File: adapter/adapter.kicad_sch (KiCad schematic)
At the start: 13 parts, among them J1 AudioJack4, J2 AudioJack4, J3 Conn_01x02_Female, J4 Conn_01x03_Female, J5 Conn_01x03_Female, J6 Conn_01x02_Female, J7 Conn_01x06_Female, J9 Conn_01x06_Female, SW1 SW_SPST, SW2 SW_SPST, U1 eliteC, U2 eliteC, U3 YAAJ_WeAct_BlackPill_Part_Lik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

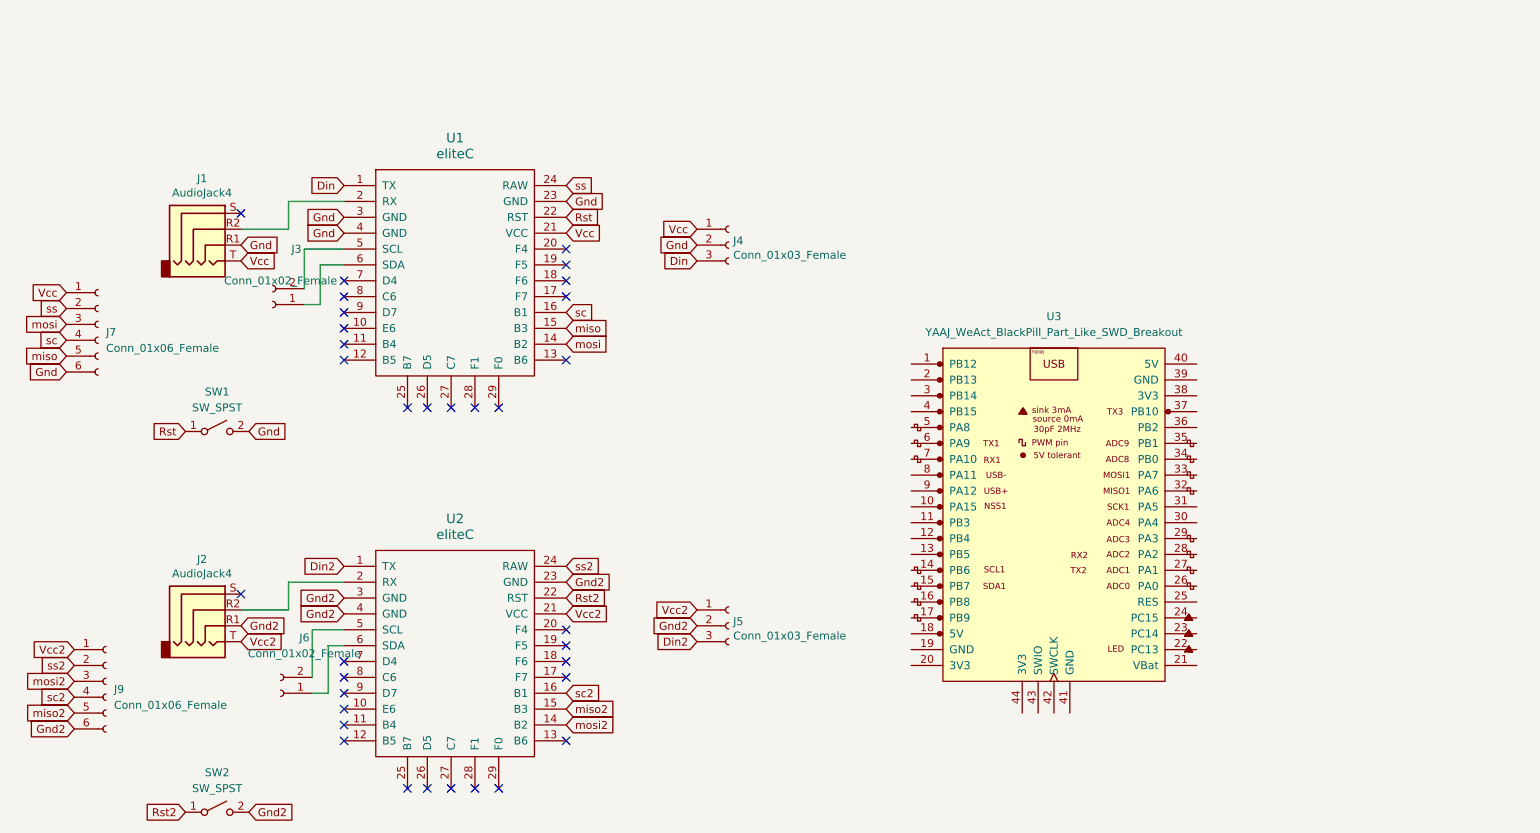
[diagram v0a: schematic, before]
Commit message: pinout
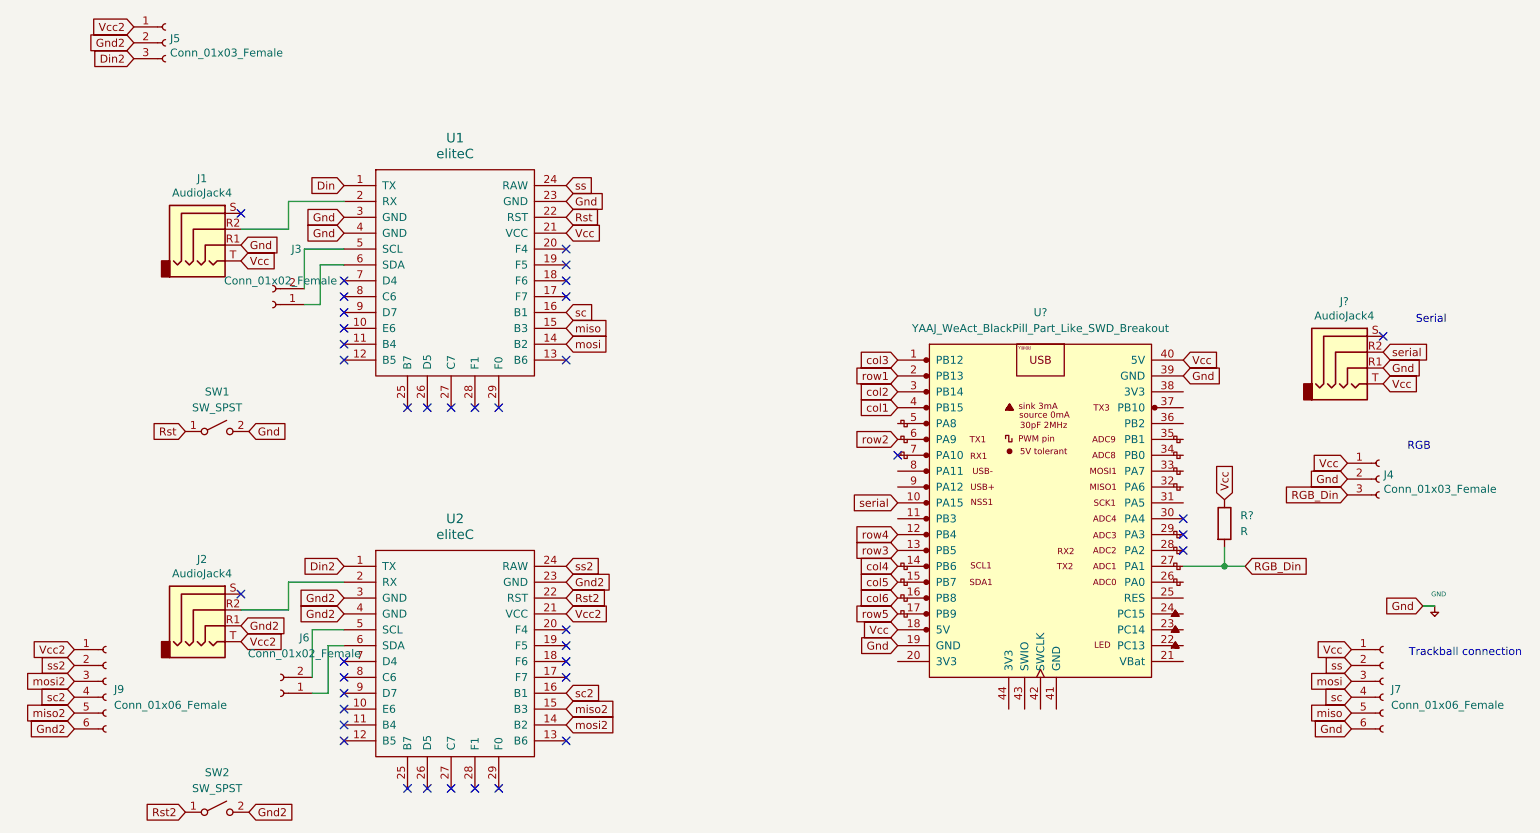
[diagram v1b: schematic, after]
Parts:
- removed U3: YAAJ_WeAct_BlackPill_Part_Like_SWD_Breakout, Library:YAAJ_WeAct_BlackPill_SWD_2, symbol YAAJ_WeAct_BlackPill_Part_Like_SWD_Breakout:YAAJ_WeAct_BlackPill_Part_Like_SWD_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
- added J?: AudioJack4, Library:Jack_3.5mm_PJ320E_Horizontal, symbol Connector:AudioJack4
- added R?: R, symbol Device:R
- added U?: YAAJ_WeAct_BlackPill_Part_Like_SWD_Breakout, Library:YAAJ_WeAct_BlackPill_SWD_2, symbol YAAJ_WeAct_BlackPill_Part_Like_SWD_Breakout:YAAJ_WeAct_BlackPill_Part_Like_SWD_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
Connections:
- net Din: no longer J4.3 (Pin_3)
- net Vcc: now also J?.T, R?.1, U?.18 (5V), U?.40 (5V)
- net Gnd renamed +5V
- net +5V: now also J?.R1, U?.19 (GND), U?.39 (GND)
- new net RGB_Din: J4.3 (Pin_3), R?.2, U?.27 (PA1)
- new net col1: U?.4 (PB15)
- new net col2: U?.3 (PB14)
- new net col3: U?.1 (PB12)
- new net col4: U?.14 (PB6)
- new net col5: U?.15 (PB7)
- new net col6: U?.16 (PB8)
- new net row1: U?.2 (PB13)
- new net row2: U?.6 (PA9)
- new net row3: U?.13 (PB5)
- new net row4: U?.12 (PB4)
- new net row5: U?.17 (PB9)
- new net serial: J?.R2, U?.10 (PA15)
- no-connect marks 34 -> 39
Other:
- note added: "RGB"
- note added: "Serial"
- note added: "Trackball connection"
- moved on the sheet: J4, J5, J7
